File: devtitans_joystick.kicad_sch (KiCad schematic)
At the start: 25 parts, among them SW1 B, SW2 Y, SW3 SELECT, SW4 START, SW5 A, SW6 X, U1 ESP32DevKitv1

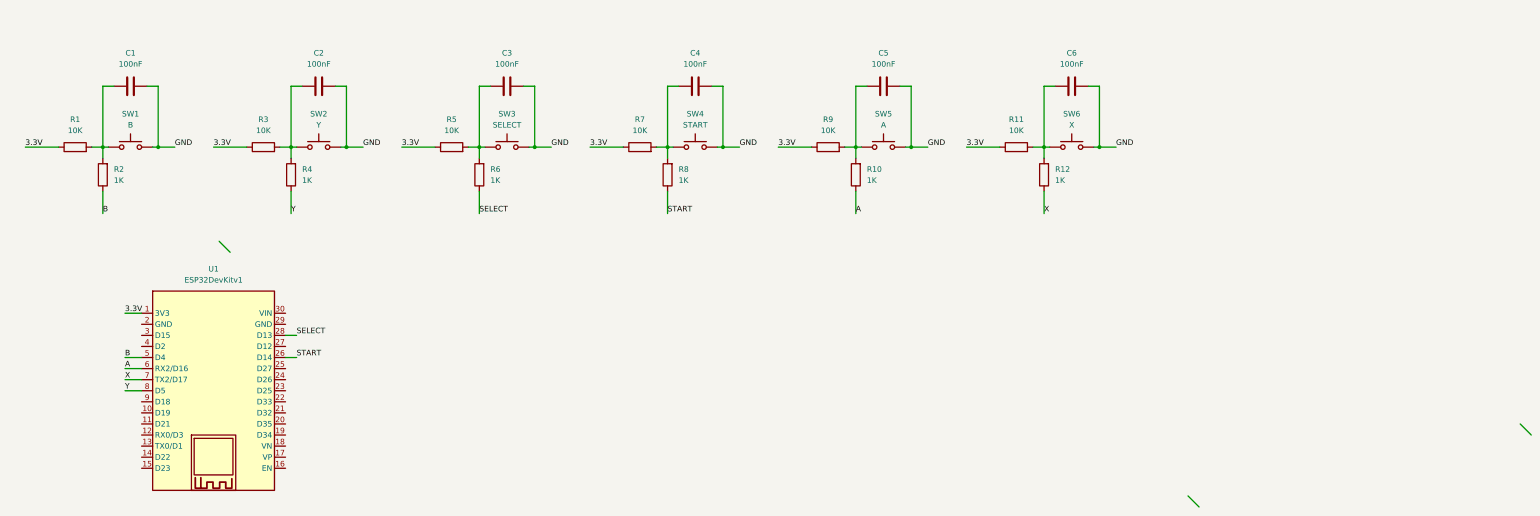
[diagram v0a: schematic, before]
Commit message: joystick snes bluetooth version with script to debug
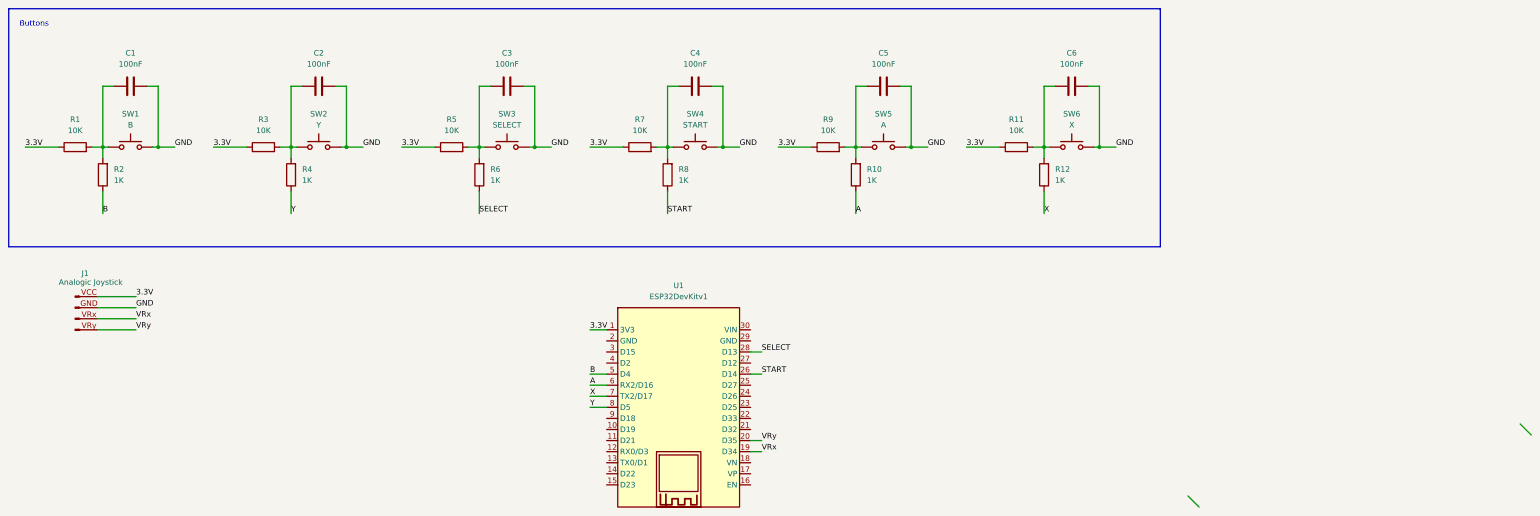
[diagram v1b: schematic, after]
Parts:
- added J1: Analogic Joystick, symbol Connector:Conn_01x04_Pin
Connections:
- net 3.3V: now also J1.VCC (Pin_1)
- net GND: now also J1.GND (Pin_2)
- net VRx: now reaches U1.19 (D34)
- net VRx: now also J1.VRx (Pin_3)
- net VRy: now reaches U1.20 (D35)
- net VRy: now also J1.VRy (Pin_4)
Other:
- note added: "Buttons"
- moved on the sheet: U1
